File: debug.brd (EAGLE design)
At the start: 120 x 50 mm, 37 parts, among them CN1 2X10 HEADER, CN2 JTAG PROG, CN3 50 PIN 0.5MM, CN4 MICRO USB B, CN5 2X10 HEADER, CN6 MICRO USB B, CN7 MICRO USB B, CN8 2X4_HEADER, Q1 MMBT3904, Q2 MMBT3904, Q3 2N7002, U1 USBLC6-2SC6, U2 USBLC6-2SC6, U3 FT231X, U4 FT231X, U5 USBLC6-2SC6, U6 FT231X

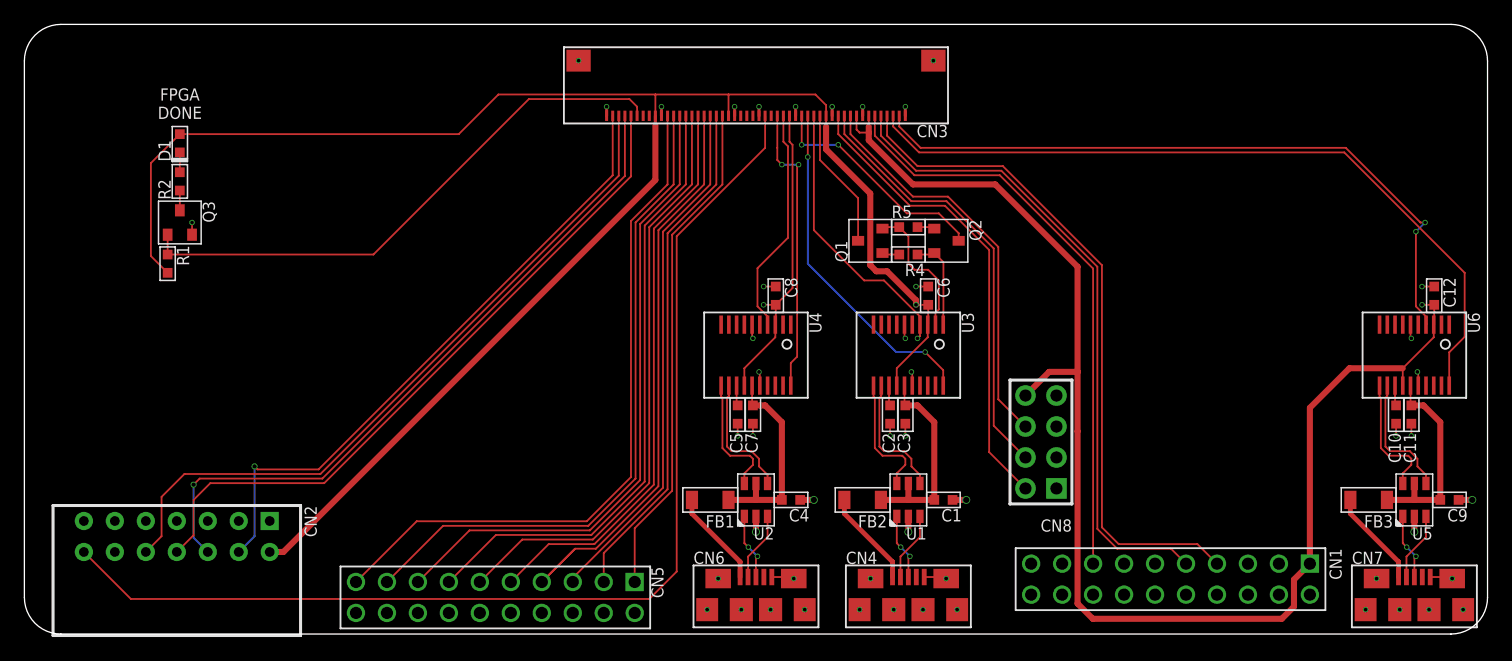
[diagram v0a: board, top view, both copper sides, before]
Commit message: Debug and power board ready for outputs
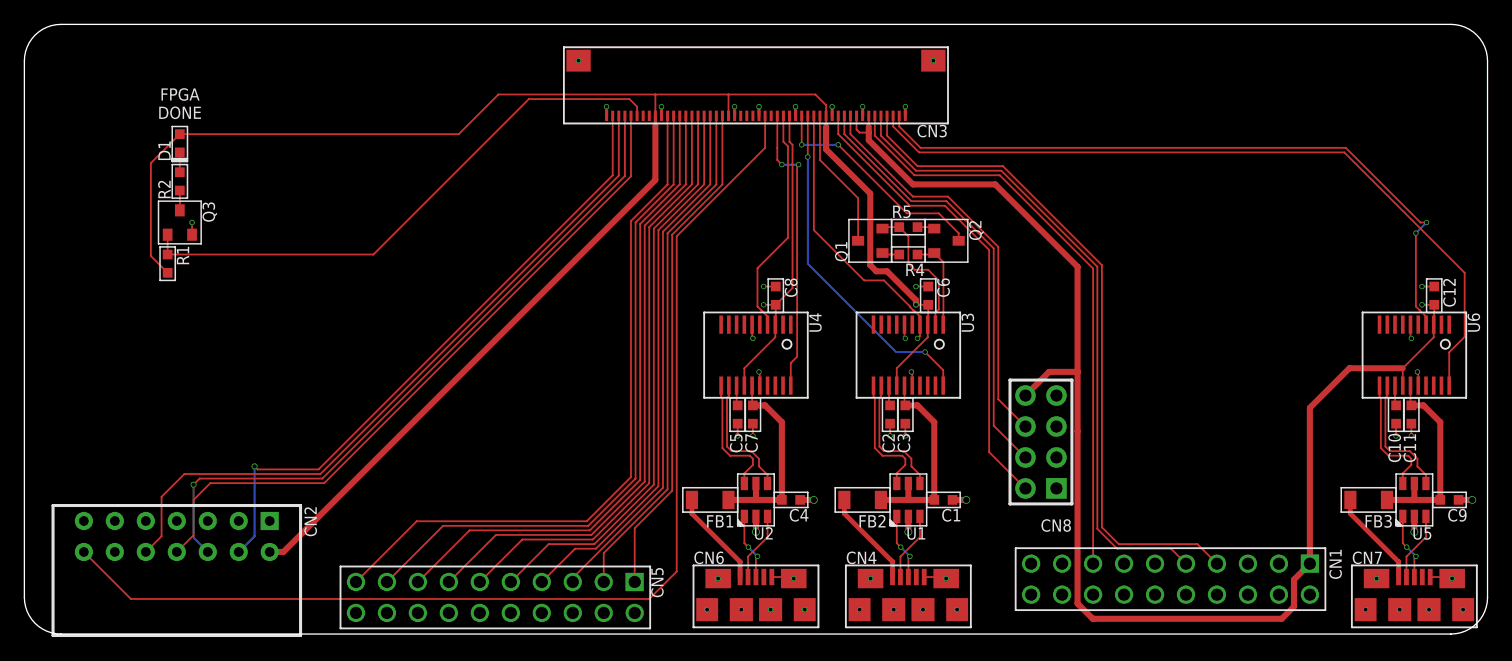
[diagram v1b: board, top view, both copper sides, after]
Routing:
- net FPGA_DEBUG_D6: track 48.5 -> 44.7 mm
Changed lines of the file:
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@@
 <wire x1="-4.25" y1="11.875" x2="-4.25" y2="17.5" width="0.15" layer="1"/>
 <wire x1="-8" y1="8.125" x2="-4.25" y2="11.875" width="0.15" layer="1"/>
-<wire x1="-17.565" y1="-20.73" x2="-14.885" y2="-18.05" width="0.15" layer="1"/>
 <wire x1="-17.565" y1="-20.73" x2="-14.835" y2="-18" width="0.15" layer="1"/>
 <wire x1="-14.835" y1="-18" x2="-13.125" y2="-18" width="0.15" layer="1"/>
@@
 <wire x1="8.875" y1="4" x2="4.75" y2="8.125" width="0.15" layer="1"/>
 <wire x1="4.75" y1="8.125" x2="4.75" y2="17.5" width="0.15" layer="1"/>
-<wire x1="13.4525" y1="1.0475" x2="10.5" y2="4" width="0.15" layer="1"/>
+<wire x1="12.975" y1="1.525" x2="12.92824375" y2="1.525" width="0.15" layer="1"/>
+<wire x1="12.92824375" y1="1.525" x2="12.65" y2="1.80324375" width="0.15" layer="1"/>
+<wire x1="12.65" y1="1.80324375" x2="12.65" y2="1.85" width="0.15" layer="1"/>
+<wire x1="13.4525" y1="1.0475" x2="12.975" y2="1.525" width="0.15" layer="1"/>
+<wire x1="12.65" y1="1.85" x2="10.5" y2="4" width="0.15" layer="1"/>
 </signal>
 <signal name="ESP32_UART_RX">
@@
 <contactref element="U4" pad="4"/>
 <wire x1="0.9525" y1="0.375" x2="0.9525" y2="1.0475" width="0.15" layer="1"/>
-<wire x1="0.9525" y1="1.0475" x2="0.125" y2="1.875" width="0.15" layer="1"/>
-<wire x1="0.125" y1="1.875" x2="0.125" y2="5" width="0.15" layer="1"/>
 <wire x1="2.625" y1="15" x2="2.25" y2="15.375" width="0.15" layer="1"/>
 <wire x1="2.25" y1="15.375" x2="2.25" y2="17.5" width="0.15" layer="1"/>
 <wire x1="0.125" y1="5" x2="2.625" y2="7.5" width="0.15" layer="1"/>
 <wire x1="2.625" y1="7.5" x2="2.625" y2="15" width="0.15" layer="1"/>
+<wire x1="0.4512" y1="1.5488" x2="0.43810625" y2="1.5488" width="0.15" layer="1"/>
+<wire x1="0.43810625" y1="1.5488" x2="0.125" y2="1.86190625" width="0.15" layer="1"/>
+<wire x1="0.9525" y1="1.0475" x2="0.4512" y2="1.5488" width="0.15" layer="1"/>
+<wire x1="0.125" y1="1.86190625" x2="0.125" y2="5" width="0.15" layer="1"/>
 </signal>
 <signal name="PMC_UART_TX">
@@
 <wire x1="11.75" y1="17.5" x2="11.75" y2="16.625" width="0.15" layer="1"/>
 <wire x1="48.375" y1="14.875" x2="54.5" y2="8.75" width="0.15" layer="1"/>
-<wire x1="54.5" y1="8.75" x2="54.875" y2="8.75" width="0.15" layer="1"/>
-<via x="54.875" y="8.75" extent="1-16" drill="0.3"/>
-<wire x1="54.875" y1="8.75" x2="54.125" y2="8" width="0.15" layer="16"/>
-<via x="54.125" y="8" extent="1-16" drill="0.3"/>
-<wire x1="54.125" y1="1.875" x2="55" y2="1" width="0.15" layer="1"/>
-<wire x1="55" y1="1" x2="55" y2="0.4225" width="0.15" layer="1"/>
+<wire x1="54.5" y1="8.75" x2="55" y2="8.75" width="0.15" layer="1"/>
+<via x="55" y="8.75" extent="1-16" drill="0.3"/>
+<wire x1="55" y1="8.75" x2="54.125" y2="7.875" width="0.15" layer="16"/>
+<via x="54.125" y="7.875" extent="1-16" drill="0.3"/>
+<wire x1="55" y1="0.4225" x2="55" y2="1" width="0.15" layer="1"/>
 <wire x1="55" y1="0.4225" x2="54.9525" y2="0.375" width="0.15" layer="1"/>
 <wire x1="11.75" y1="16.625" x2="13.5" y2="14.875" width="0.15" layer="1"/>
 <wire x1="13.5" y1="14.875" x2="48.375" y2="14.875" width="0.15" layer="1"/>
-<wire x1="54.125" y1="8" x2="54.125" y2="1.875" width="0.15" layer="1"/>
+<wire x1="54.4512" y1="1.5488" x2="54.43810625" y2="1.5488" width="0.15" layer="1"/>
+<wire x1="54.43810625" y1="1.5488" x2="54.125" y2="1.86190625" width="0.15" layer="1"/>
+<wire x1="55" y1="1" x2="54.4512" y2="1.5488" width="0.15" layer="1"/>
+<wire x1="54.125" y1="1.86190625" x2="54.125" y2="7.875" width="0.15" layer="1"/>
 </signal>
 <signal name="PMC_UART_RX">
@@
 <wire x1="8.5" y1="16.125" x2="9.25" y2="16.125" width="0.15" layer="1"/>
 <contactref element="CN8" pad="5"/>
-<wire x1="26.27" y1="-8.48" x2="26.375" y2="-8.375" width="0.15" layer="1"/>
 <wire x1="22.105" y1="-5.44" x2="24.045" y2="-3.5" width="0.5" layer="1"/>
 <wire x1="24.045" y1="-3.5" x2="26.375" y2="-3.5" width="0.5" layer="1"/>
